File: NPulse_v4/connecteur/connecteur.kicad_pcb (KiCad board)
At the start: 4 copper layers, 39.8 x 44 mm, 75 parts, among them J1 Conn_01x01, J10 Conn_02x05_Odd_Even, J11 Conn_01x01, J12 Conn_01x01, J13 Conn_02x05_Odd_Even, J14 Conn_01x01, J15 Conn_01x01, J16 Conn_01x01, J17 Conn_01x01, J18 Conn_01x01, J19 Conn_01x01, J2 Conn_01x01, J20 Conn_01x01, J21 Conn_01x01, J22 Conn_01x01, J23 Conn_01x01, J25 Conn_01x01, J26 Conn_01x01, J27 Conn_01x01, J29 Conn_01x01, J3 Conn_01x01, J30 Conn_01x01, J32 Conn_02x05_Odd_Even, J34 Conn_01x01, J35 Conn_02x05_Odd_Even, J36 Conn_01x01, J37 Conn_01x01, J38 Conn_01x01, J39 Conn_01x01, J4 Conn_01x01, J40 Conn_01x01, J41 Conn_01x01, J42 Conn_01x01, J43 Conn_01x01, J44 Conn_01x01, J45 Conn_01x01, J46 Conn_01x01, J47 Conn_01x01, J48 Conn_01x01, J49 Conn_01x01, J5 Conn_01x01, J50 Conn_01x01, J51 Conn_01x01, J52 Conn_01x01, J53 Conn_01x01, J54 Conn_02x05_Odd_Even, J55 Conn_01x01, J56 Conn_01x01, J57 Conn_02x05_Odd_Even, J58 Conn_01x01, J59 Conn_01x01, J6 Conn_01x01, J60 Conn_01x01, J61 Conn_01x01, J62 Conn_01x01, J63 Conn_01x01, J64 Conn_01x01, J65 Conn_01x01, J66 Conn_01x01, J67 Conn_01x01, J68 Conn_01x01, J69 Conn_01x01, J7 Conn_01x01, J70 Conn_01x01, J72 Conn_01x01, J73 Conn_01x01, J74 Conn_01x01, J75 Conn_01x01, J76 Conn_01x01, J77 Conn_01x01, J8 Conn_01x01, J9 Conn_01x01

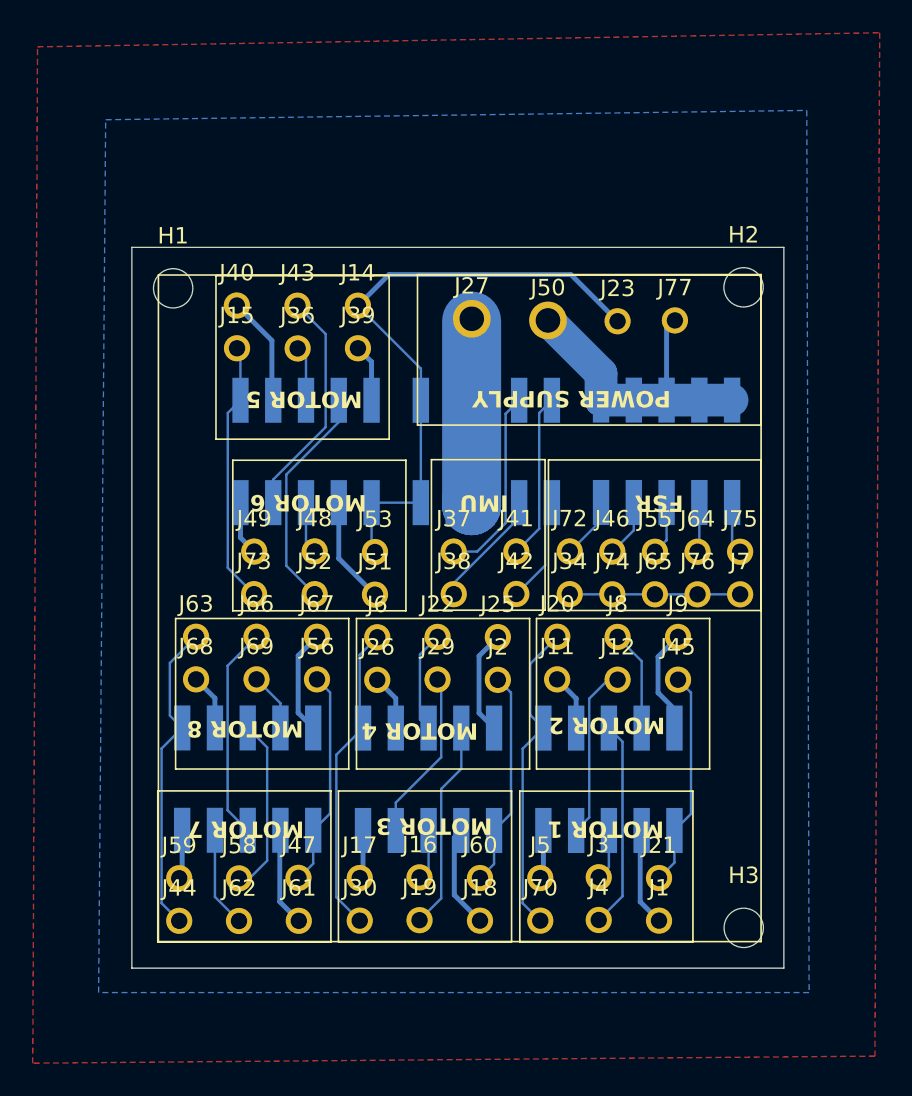
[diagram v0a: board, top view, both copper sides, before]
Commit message: generate gerber files
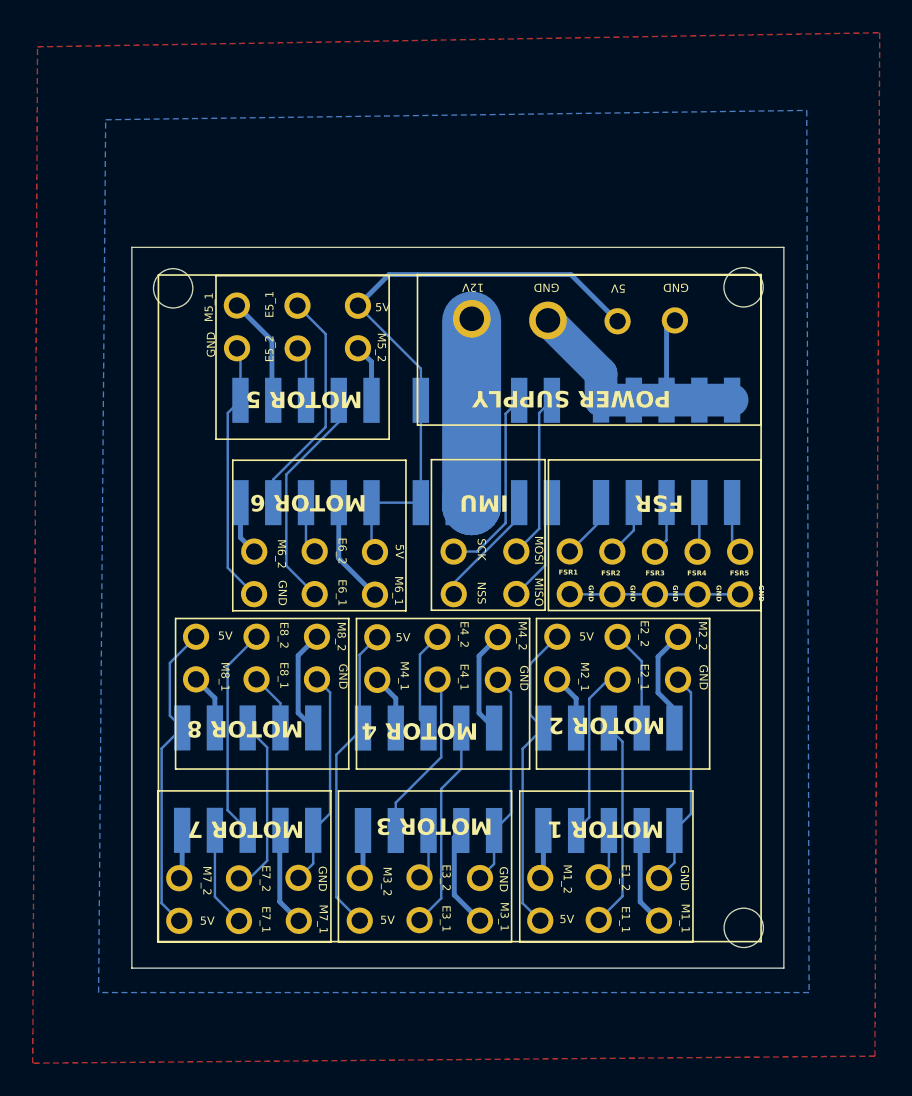
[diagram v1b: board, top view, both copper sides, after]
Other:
- board text added: "12V"
- board text added: "5V"
- board text added: "E1_1"
- board text added: "E1_2"
- board text added: "E2_1"
- board text added: "E2_2"
- board text added: "E3_1"
- board text added: "E3_2"
- board text added: "E4_1"
- board text added: "E4_2"
- board text added: "E5_1"
- board text added: "E5_2"
- board text added: "E6_1"
- board text added: "E6_2"
- board text added: "E7_1"
- board text added: "E7_2"
- board text added: "E8_1"
- board text added: "E8_2"
- board text added: "FSR1"
- board text added: "FSR2"
- board text added: "FSR3"
- board text added: "FSR4"
- board text added: "FSR5"
- board text added: "GND"
- board text added: "M1_1"
- board text added: "M1_2"
- board text added: "M2_1"
- board text added: "M2_2"
- board text added: "M3_1"
- board text added: "M3_2"
- board text added: "M4_1"
- board text added: "M4_2"
- board text added: "M5_1"
- board text added: "M5_2"
- board text added: "M6_1"
- board text added: "M6_2"
- board text added: "M7_1"
- board text added: "M7_2"
- board text added: "M8_1"
- board text added: "M8_2"
- board text added: "MISO"
- board text added: "MOSI"
- board text added: "NSS"
- board text added: "SCK"
